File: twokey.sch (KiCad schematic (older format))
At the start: 12 parts, among them J1 12401610E4#2A, SW1 SW_SPST, SW2 SW_SPST, U1 ATSAMD21E18A-A, U2 MCP1700-3302E_SOT23

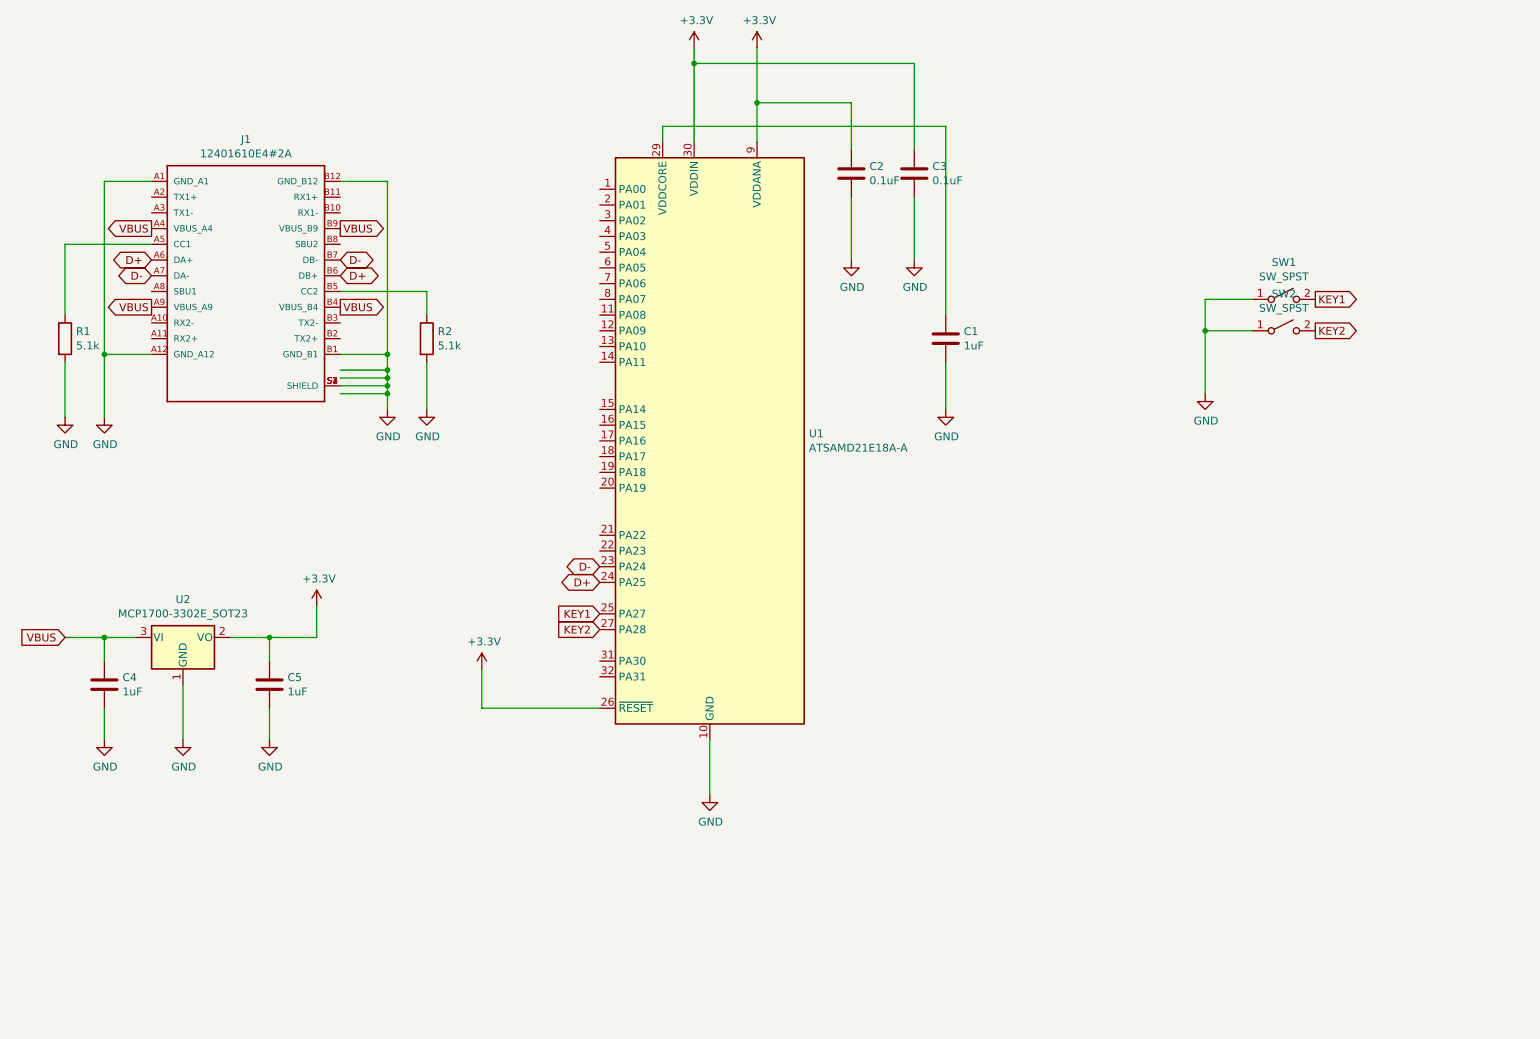
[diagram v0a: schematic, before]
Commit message: ordered pcb
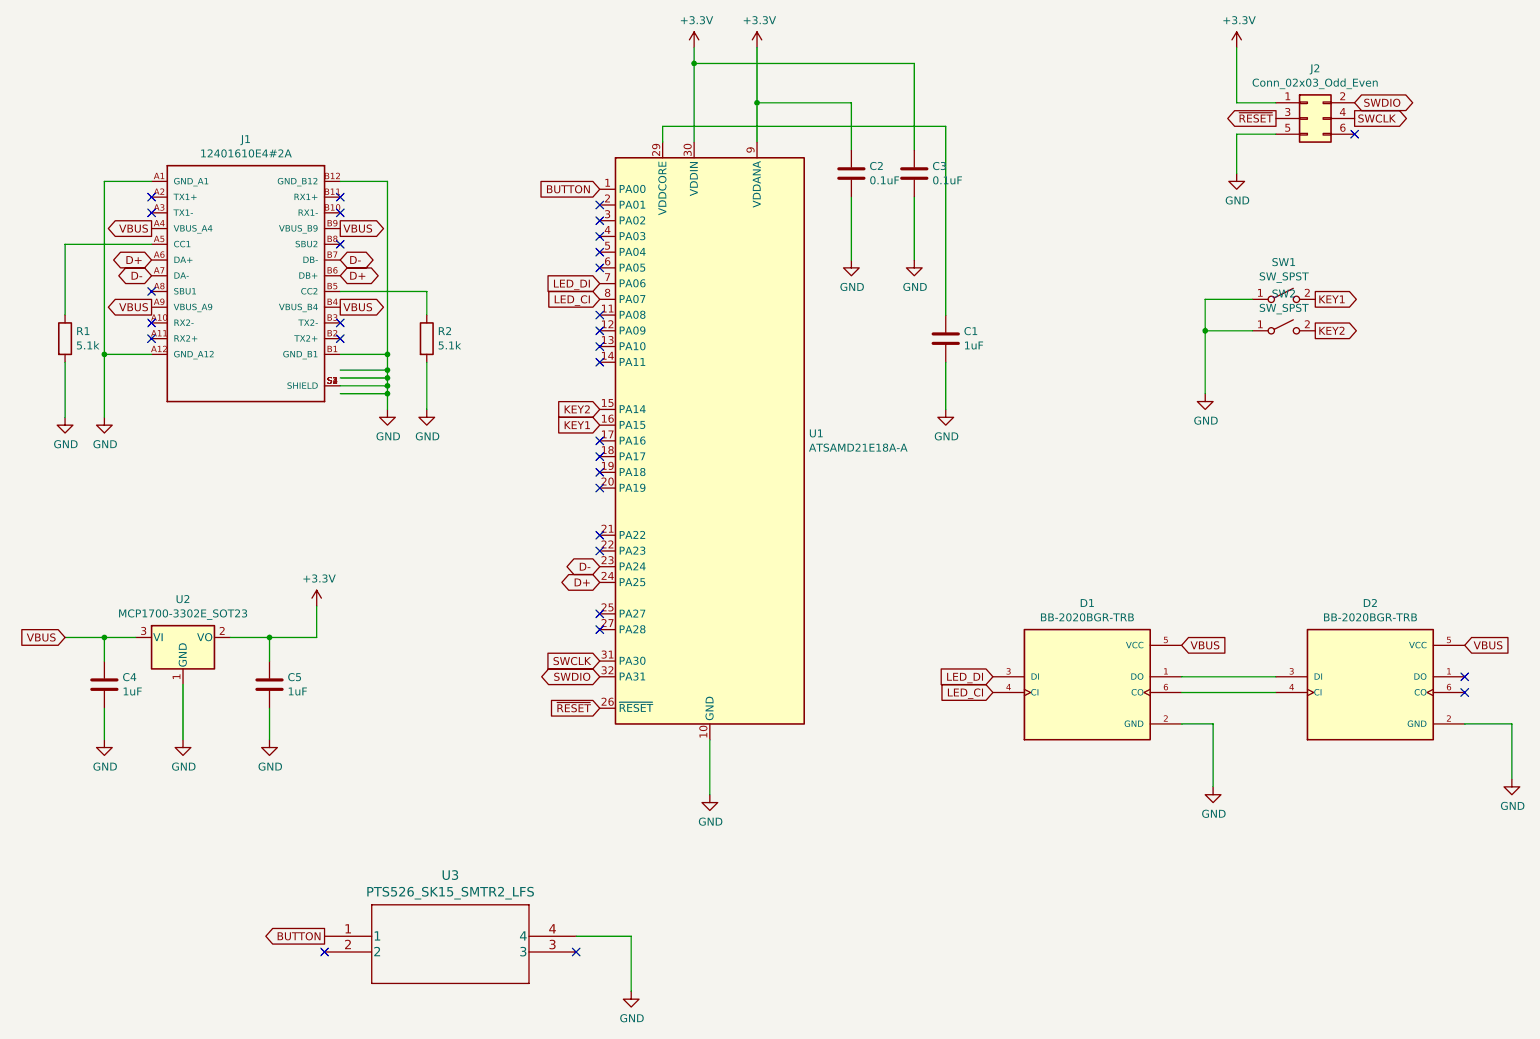
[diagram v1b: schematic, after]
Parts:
- added D1, D2: BB-2020BGR-TRB, twokey:LED_BB-2020BGR-TRB, symbol BB-2020BGR-TRB:BB-2020BGR-TRB
- added J2: Conn_02x03_Odd_Even, twokey:TC2030-IDC-NL, symbol Connector_Generic:Conn_02x03_Odd_Even
- added U3: PTS526_SK15_SMTR2_LFS, twokey:PTS526 SK15 SMTR2 LFS, symbol 2021-07-27_21-35-03:PTS526_SK15_SMTR2_LFS
- U1: footprint Package_QFP:TQFP-32_7x7mm_P0.8mm -> Package_DFN_QFN:QFN-32-1EP_5x5mm_P0.5mm_EP3.6x3.6mm
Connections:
- net labels added: BUTTON, LED_CI, LED_DI, SWCLK, SWDIO, ~RESET
- wire segments 53 -> 63
- no-connect marks 0 -> 32
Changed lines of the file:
@@
 F 0 "U1" H 6130 3696 50  0000 L CNN
 F 1 "ATSAMD21E18A-A" H 6130 3605 50  0000 L CNN
-F 2 "Package_QFP:TQFP-32_7x7mm_P0.8mm" H 6400 1800 50  0001 C CNN
+F 2 "Package_DFN_QFN:QFN-32-1EP_5x5mm_P0.5mm_EP3.6x3.6mm" H 6400 1800 50  0001 C CNN
 F 3 "http://ww1.microchip.com/downloads/en/DeviceDoc/SAM_D21_DA1_Family_Data%20Sheet_DS40001882E.pdf" H 5500 3650 50  0001 C CNN
 	1    5500 3650
@@
 Wire Wire Line
 	7000 3150 7000 3450
-$Comp
-L power:+3.3V #PWR04
-U 1 1 60F4548C
-P 4050 5100
-F 0 "#PWR04" H 4050 4950 50  0001 C CNN
-F 1 "+3.3V" H 4065 5273 50  0000 C CNN
-F 2 "" H 4050 5100 50  0001 C CNN
-F 3 "" H 4050 5100 50  0001 C CNN
-	1    4050 5100
-	1    0    0    -1
-$EndComp
-Wire Wire Line
-	4050 5100 4050 5350
-Wire Wire Line
-	4050 5350 4800 5350
 $Comp
 L Device:C C2
@@
 	1    0    0    -1
 $EndComp
-Text GLabel 4800 4750 0    50   Input ~ 0
-KEY1
-Text GLabel 4800 4850 0    50   Input ~ 0
-KEY2
 Text GLabel 9350 2750 2    50   Output ~ 0
 KEY1
@@
 Wire Wire Line
 	8650 2950 8650 3350
+$Comp
+L BB-2020BGR-TRB:BB-2020BGR-TRB D1
+U 1 1 6100A1F5
+P 7900 5250
+F 0 "D1" H 7900 5817 50  0000 C CNN
+F 1 "BB-2020BGR-TRB" H 7900 5726 50  0000 C CNN
+F 2 "twokey:LED_BB-2020BGR-TRB" H 7900 5250 50  0001 L BNN
+F 3 "" H 7900 5250 50  0001 L BNN
+F 4 "--" H 7900 5250 50  0001 L BNN "PARTREV"
+F 5 "American Bright LED" H 7900 5250 50  0001 L BNN "MANUFACTURER"
+F 6 "0.75mm" H 7900 5250 50  0001 L BNN "MAXIMUM_PACKAGE_HEIGHT"
+F 7 "Manufacturer recommendations" H 7900 5250 50  0001 L BNN "STANDARD"
+	1    7900 5250
+	1    0    0    -1
+$EndComp
+$Comp
+L Connector_Generic:Conn_02x03_Odd_Even J2
+U 1 1 610124D7
+P 9300 1600
+F 0 "J2" H 9350 1917 50  0000 C CNN
+F 1 "Conn_02x03_Odd_Even" H 9350 1826 50  0000 C CNN
+F 2 "twokey:TC2030-IDC-NL" H 9300 1600 50  0001 C CNN
+F 3 "~" H 9300 1600 50  0001 C CNN
+	1    9300 1600
+	1    0    0    -1
+$EndComp
+$Comp
+L power:GND #PWR019
+U 1 1 61013843
+P 8850 1950
+F 0 "#PWR019" H 8850 1700 50  0001 C CNN
+F 1 "GND" H 8855 1777 50  0000 C CNN
+F 2 "" H 8850 1950 50  0001 C CNN
+F 3 "" H 8850 1950 50  0001 C CNN
+	1    8850 1950
+	1    0    0    -1
+$EndComp
+Wire Wire Line
+	9100 1700 8850 1700
+Wire Wire Line
+	8850 1700 8850 1950
+$Comp
+L power:+3.3V #PWR018
+U 1 1 610159A3
+P 8850 1150
+F 0 "#PWR018" H 8850 1000 50  0001 C CNN
+F 1 "+3.3V" H 8865 1323 50  0000 C CNN
+F 2 "" H 8850 1150 50  0001 C CNN
+F 3 "" H 8850 1150 50  0001 C CNN
+	1    8850 1150
+	1    0    0    -1
+$EndComp
+Wire Wire Line
+	8850 1150 8850 1500
+Wire Wire Line
+	8850 1500 9100 1500
+Text GLabel 9100 1600 0    50   Output ~ 0
+~RESET
+Text GLabel 4800 5350 0    50   Input ~ 0
+~RESET
+Text GLabel 4800 5150 0    50   BiDi ~ 0
+SWDIO
+Text GLabel 9600 1500 2    50   BiDi ~ 0
+SWDIO
+Text GLabel 9600 1600 2    50   Output ~ 0
+SWCLK
+Text GLabel 4800 5050 0    50   Input ~ 0
+SWCLK
+NoConn ~ 9600 1700
+NoConn ~ 4800 2150
+NoConn ~ 4800 2250
+NoConn ~ 4800 2350
+NoConn ~ 4800 2450
+NoConn ~ 4800 2550
+NoConn ~ 4800 2950
+NoConn ~ 4800 3050
+NoConn ~ 4800 3150
+NoConn ~ 4800 3650
+NoConn ~ 4800 3750
+NoConn ~ 4800 3850
+NoConn ~ 4800 3950
+NoConn ~ 4800 4250
+NoConn ~ 4800 4350
+NoConn ~ 1950 3000
+NoConn ~ 1950 2700
+NoConn ~ 1950 2900
+NoConn ~ 1950 2200
+NoConn ~ 1950 2100
+NoConn ~ 3150 2100
+NoConn ~ 3150 2200
+NoConn ~ 3150 2400
+NoConn ~ 3150 2900
+NoConn ~ 3150 3000
+$Comp
+L power:GND #PWR017
+U 1 1 6103CE75
+P 8700 5850
+F 0 "#PWR017" H 8700 5600 50  0001 C CNN
+F 1 "GND" H 8705 5677 50  0000 C CNN
+F 2 "" H 8700 5850 50  0001 C CNN
+F 3 "" H 8700 5850 50  0001 C CNN
+	1    8700 5850
+	1    0    0    -1
+$EndComp
+$Comp
+L power:GND #PWR020
+U 1 1 6103D8BF
+P 10600 5800
+F 0 "#PWR020" H 10600 5550 50  0001 C CNN
+F 1 "GND" H 10605 5627 50  0000 C CNN
+F 2 "" H 10600 5800 50  0001 C CNN
+F 3 "" H 10600 5800 50  0001 C CNN
+	1    10600 5800
+	1    0    0    -1
+$EndComp
+Wire Wire Line
+	8500 5450 8700 5450
+Wire Wire Line
+	8700 5450 8700 5850
+Wire Wire Line
+	10300 5450 10600 5450
+Wire Wire Line
+	10600 5450 10600 5800
+Text GLabel 8500 4950 2    50   Input ~ 0
+VBUS
+Text GLabel 10300 4950 2    50   Input ~ 0
+VBUS
+Wire Wire Line
+	8500 5150 9100 5150
+Wire Wire Line
+	8500 5250 9100 5250
+$Comp
+L BB-2020BGR-TRB:BB-2020BGR-TRB D2
+U 1 1 6100ACA2
+P 9700 5250
+F 0 "D2" H 9700 5817 50  0000 C CNN
+F 1 "BB-2020BGR-TRB" H 9700 5726 50  0000 C CNN
+F 2 "twokey:LED_BB-2020BGR-TRB" H 9700 5250 50  0001 L BNN
+F 3 "" H 9700 5250 50  0001 L BNN
+F 4 "--" H 9700 5250 50  0001 L BNN "PARTREV"
+F 5 "American Bright LED" H 9700 5250 50  0001 L BNN "MANUFACTURER"
+F 6 "0.75mm" H 9700 5250 50  0001 L BNN "MAXIMUM_PACKAGE_HEIGHT"
+F 7 "Manufacturer recommendations" H 9700 5250 50  0001 L BNN "STANDARD"
+	1    9700 5250
+	1    0    0    -1
+$EndComp
+NoConn ~ 10300 5150
+NoConn ~ 10300 5250
+Text GLabel 7300 5150 0    50   Input ~ 0
+LED_DI
+Text GLabel 7300 5250 0    50   Input ~ 0
+LED_CI
+$Comp
+L 2021-07-27_21-35-03:PTS526_SK15_SMTR2_LFS U3
+U 1 1 6104711C
+P 3050 6800
+F 0 "U3" H 3850 7187 60  0000 C CNN
+F 1 "PTS526_SK15_SMTR2_LFS" H 3850 7081 60  0000 C CNN
+F 2 "twokey:PTS526 SK15 SMTR2 LFS" H 3850 7040 60  0001 C CNN
+F 3 "" H 3050 6800 60  0000 C CNN
+	1    3050 6800
+	1    0    0    -1
+$EndComp
+NoConn ~ 3050 6900
+NoConn ~ 4650 6900
+Text GLabel 3050 6800 0    50   Output ~ 0
+BUTTON
+$Comp
+L power:GND #PWR04
+U 1 1 61049E96
+P 5000 7150
+F 0 "#PWR04" H 5000 6900 50  0001 C CNN
+F 1 "GND" H 5005 6977 50  0000 C CNN
+F 2 "" H 5000 7150 50  0001 C CNN
+F 3 "" H 5000 7150 50  0001 C CNN
+	1    5000 7150
+	1    0    0    -1
+$EndComp
+Wire Wire Line
+	4650 6800 5000 6800
+Wire Wire Line
+	5000 6800 5000 7150
+Text GLabel 4800 3550 0    50   Input ~ 0
+KEY1
+Text GLabel 4800 3450 0    50   Input ~ 0
+KEY2
+NoConn ~ 4800 4750
+NoConn ~ 4800 4850
+Text GLabel 4800 2650 0    50   Input ~ 0
+LED_DI
+Text GLabel 4800 2750 0    50   Input ~ 0
+LED_CI
+NoConn ~ 4800 2850
+Text GLabel 4800 2050 0    50   Input ~ 0
+BUTTON
 $EndSCHEMATC
